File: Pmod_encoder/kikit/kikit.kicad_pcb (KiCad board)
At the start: 2 copper layers, 93.2 x 99.2 mm, 416 parts, among them SW1 SW_SPDT, SW2 RotaryEncoder_Switch

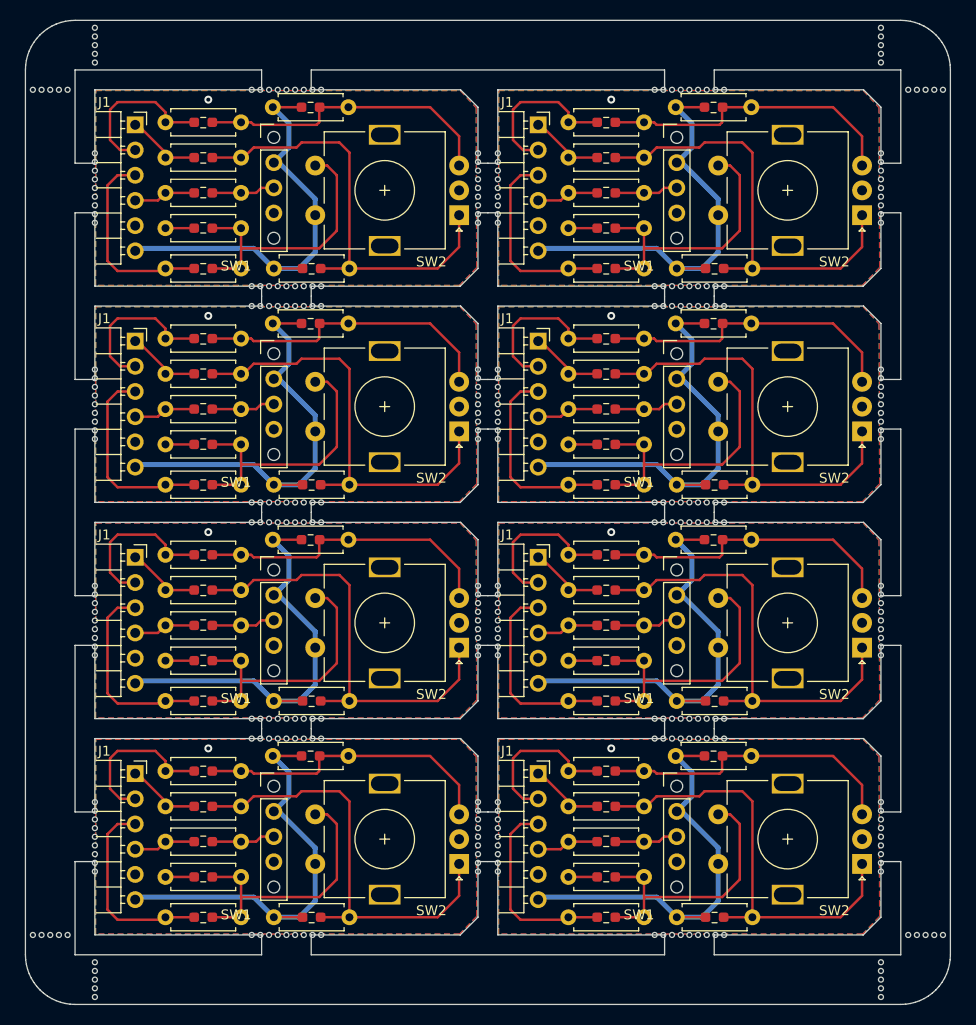
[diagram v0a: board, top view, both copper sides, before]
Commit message: 605
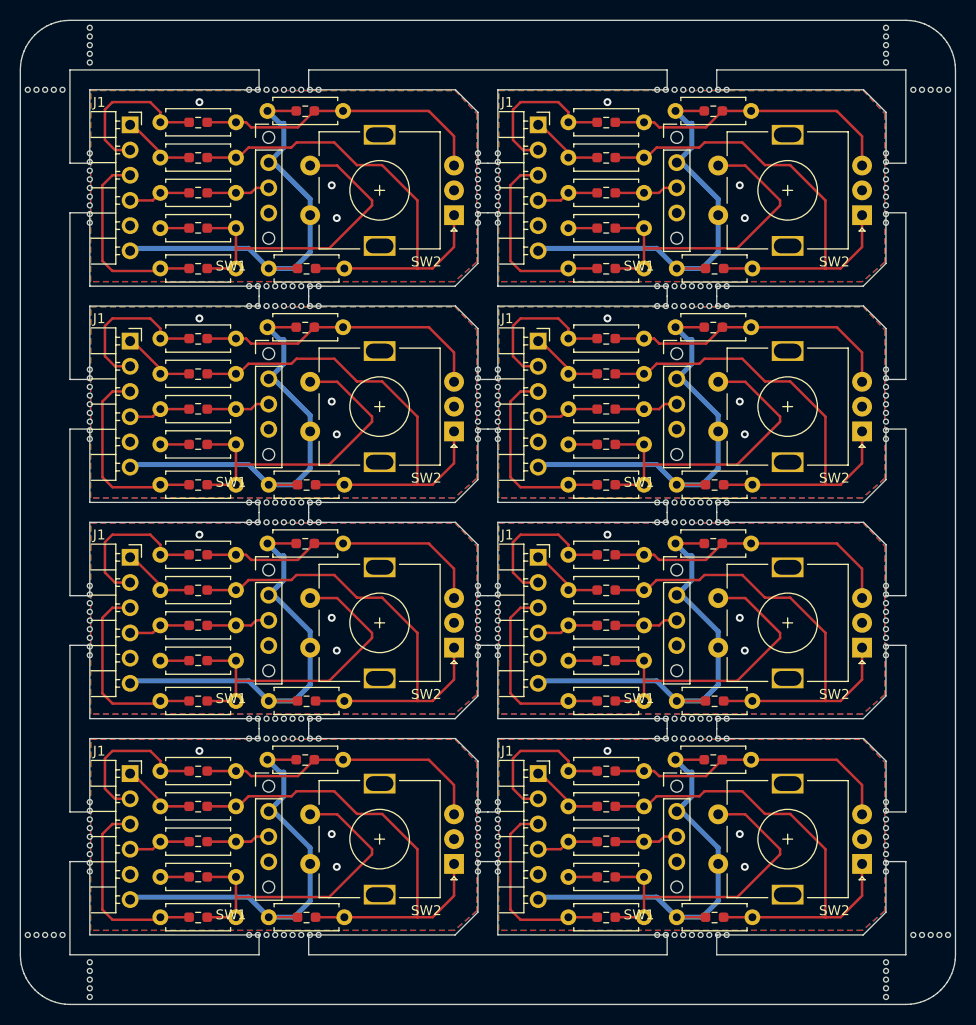
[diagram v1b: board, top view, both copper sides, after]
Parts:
- removed the G*** at (137.6, 37.1)
- removed the G*** at (137.6, 58.9)
- removed the G*** at (137.6, 102.5)
- removed the G*** at (137.6, 80.7)
- removed the J1 at (113.0, 95.9)
- removed the J1 at (113.0, 30.5)
- removed the J1 at (113.0, 52.3)
- removed the J1 at (113.0, 74.1)
- removed the R1 at (123.6, 37.4)
- removed the R1 at (123.6, 81.0)
- removed the R1 at (123.6, 59.2)
- removed the R1 at (123.6, 102.8)
- removed the R2 at (116.0, 95.7)
- removed the R2 at (116.0, 52.1)
- removed the R2 at (116.0, 30.3)
- removed the R2 at (116.0, 73.9)
- removed the R3 at (116.0, 99.2)
- removed the R3 at (116.0, 33.8)
- removed the R3 at (116.0, 55.6)
- removed the R3 at (116.0, 77.4)
- removed the R4 at (116.0, 110.4)
- removed the R4 at (116.0, 88.6)
- removed the R4 at (116.0, 45.0)
- removed the R4 at (116.0, 66.8)
- removed the R5 at (167.4, 28.8)
- removed the R5 at (126.8, 94.1)
- removed the R5 at (126.8, 72.3)
- removed the R5 at (167.4, 72.3)
- removed the R5 at (126.8, 50.5)
- removed the R5 at (167.4, 94.1)
- removed the R5 at (126.8, 28.8)
- removed the R5 at (167.4, 50.5)
- removed the R6 at (123.6, 106.3)
- removed the R6 at (123.6, 84.5)
- removed the R6 at (123.6, 40.9)
- removed the R6 at (123.6, 62.7)
- removed the R7 at (126.9, 45.0)
- removed the R7 at (126.9, 110.4)
- removed the R7 at (126.9, 66.8)
- removed the R7 at (126.9, 88.6)
- removed the REF** at (168.8, 68.6)
- removed the REF** at (124.7, 68.6)
- removed the REF** at (168.8, 27.0)
- removed the REF** at (168.8, 48.8)
- removed the REF** at (147.5, 84.0)
- removed the REF** at (165.3, 27.0)
- removed the REF** at (125.6, 27.0)
- removed the REF** at (147.5, 34.3)
- removed the REF** at (147.5, 77.0)
- removed the REF** at (188.1, 101.4)
- removed the REF** at (172.3, 90.4)
- removed the REF** at (188.1, 38.6)
- removed the REF** at (108.9, 40.4)
- removed the REF** at (128.2, 112.2)
- removed the REF** at (167.1, 68.6)
- removed the REF** at (147.5, 37.8)
- removed the REF** at (188.1, 40.4)
- removed the REF** at (191.7, 112.2)
- removed the REF** at (169.7, 68.6)
- removed the REF** at (126.4, 48.8)
- removed the REF** at (147.5, 104.0)
- removed the REF** at (125.6, 70.6)
- removed the REF** at (165.3, 68.6)
- removed the REF** at (127.3, 112.2)
- removed the REF** at (129.1, 70.6)
- removed the REF** at (172.3, 70.6)
- removed the REF** at (131.7, 27.0)
- removed the REF** at (131.7, 112.2)
- removed the REF** at (166.2, 92.4)
- removed the REF** at (191.7, 27.0)
- removed the REF** at (188.1, 81.4)
- removed the REF** at (108.9, 34.3)
- removed the REF** at (188.1, 56.1)
- removed the REF** at (125.6, 48.8)
- removed the REF** at (102.6, 112.2)
- removed the REF** at (124.7, 27.0)
- removed the REF** at (108.9, 59.6)
- removed the REF** at (108.9, 84.0)
- removed the REF** at (171.4, 48.8)
- removed the REF** at (147.5, 62.2)
- removed the REF** at (147.5, 36.9)
- removed the REF** at (165.3, 92.4)
- removed the REF** at (129.9, 92.4)
- removed the REF** at (188.1, 24.2)
- removed the REF** at (167.9, 46.8)
- removed the REF** at (172.3, 48.8)
- removed the REF** at (188.1, 100.5)
- removed the REF** at (147.5, 61.3)
- removed the REF** at (106.1, 112.2)
- removed the REF** at (128.2, 90.4)
- removed the REF** at (124.7, 112.2)
- removed the REF** at (108.9, 56.9)
- removed the REF** at (165.3, 48.8)
- removed the REF** at (131.7, 90.4)
- removed the REF** at (108.9, 77.0)
- removed the REF** at (147.5, 100.5)
- removed the REF** at (147.5, 59.6)
- removed the REF** at (167.1, 92.4)
- removed the REF** at (166.2, 48.8)
- removed the REF** at (188.1, 118.4)
- removed the REF** at (131.7, 68.6)
- removed the REF** at (124.7, 90.4)
- removed the REF** at (188.1, 62.2)
- removed the REF** at (166.2, 27.0)
- removed the REF** at (108.9, 117.6)
- removed the REF** at (108.9, 57.8)
- removed the REF** at (167.9, 27.0)
- removed the REF** at (147.5, 80.5)
- removed the REF** at (167.9, 48.8)
- removed the REF** at (129.9, 46.8)
- removed the REF** at (128.2, 68.6)
- removed the REF** at (170.6, 92.4)
- removed the REF** at (147.5, 56.9)
- removed the REF** at (147.5, 104.9)
- removed the REF** at (108.9, 101.4)
- removed the REF** at (188.1, 36.0)
- removed the REF** at (147.5, 102.3)
- removed the REF** at (188.1, 104.0)
- removed the REF** at (167.9, 68.6)
- removed the REF** at (171.4, 112.2)
- removed the REF** at (188.1, 84.0)
- removed the REF** at (108.9, 39.5)
- removed the REF** at (125.6, 112.2)
- removed the REF** at (188.1, 82.2)
- removed the REF** at (147.5, 55.2)
- removed the REF** at (129.9, 70.6)
- removed the REF** at (108.9, 78.7)
- removed the REF** at (126.4, 112.2)
- removed the REF** at (167.9, 90.4)
- removed the REF** at (108.9, 36.9)
- removed the REF** at (147.5, 101.4)
- removed the REF** at (125.6, 90.4)
- removed the REF** at (188.1, 83.1)
- removed the REF** at (128.2, 48.8)
- removed the REF** at (188.1, 115.8)
- removed the REF** at (188.1, 105.8)
- removed the REF** at (169.7, 46.8)
- removed the REF** at (168.8, 46.8)
- removed the REF** at (108.9, 115.8)
- removed the REF** at (108.9, 37.8)
- removed the REF** at (108.9, 104.9)
- removed the REF** at (131.7, 48.8)
- removed the REF** at (194.4, 27.0)
- removed the REF** at (147.5, 38.6)
- removed the REF** at (108.9, 24.2)
- removed the REF** at (188.1, 39.5)
- removed the REF** at (147.5, 83.1)
- removed the REF** at (147.5, 99.7)
- removed the REF** at (147.5, 105.8)
- removed the REF** at (108.9, 99.7)
- removed the REF** at (131.7, 46.8)
- removed the REF** at (165.3, 70.6)
- removed the REF** at (108.9, 55.2)
- removed the REF** at (127.3, 68.6)
- removed the REF** at (194.4, 112.2)
- removed the REF** at (108.9, 60.4)
- removed the REF** at (188.1, 99.7)
- removed the REF** at (167.9, 112.2)
- removed the REF** at (105.3, 112.2)
- removed the REF** at (166.2, 46.8)
- removed the REF** at (129.9, 90.4)
- removed the REF** at (129.9, 48.8)
- removed the REF** at (170.6, 48.8)
- removed the REF** at (188.1, 59.6)
- removed the REF** at (168.8, 92.4)
- removed the REF** at (165.3, 90.4)
- removed the REF** at (129.1, 48.8)
- removed the REF** at (166.2, 68.6)
- removed the REF** at (147.5, 36.0)
- removed the REF** at (108.9, 22.5)
- removed the REF** at (129.1, 68.6)
- removed the REF** at (193.5, 27.0)
- removed the REF** at (188.1, 78.7)
- removed the REF** at (108.9, 116.7)
- removed the REF** at (170.6, 112.2)
- removed the REF** at (108.9, 102.3)
- removed the REF** at (108.9, 21.6)
- removed the REF** at (129.9, 27.0)
- removed the REF** at (165.3, 112.2)
- removed the REF** at (167.9, 92.4)
- removed the REF** at (171.4, 68.6)
- removed the REF** at (108.9, 118.4)
- removed the REF** at (130.8, 48.8)
- removed the REF** at (166.2, 70.6)
- removed the REF** at (108.9, 38.6)
- removed the REF** at (108.9, 61.3)
- removed the REF** at (171.4, 70.6)
- removed the REF** at (167.1, 46.8)
- removed the REF** at (188.1, 61.3)
- removed the REF** at (131.7, 70.6)
- removed the REF** at (169.7, 48.8)
- removed the REF** at (128.2, 70.6)
- removed the REF** at (167.9, 70.6)
- removed the REF** at (108.9, 56.1)
- removed the REF** at (108.9, 58.7)
- removed the REF** at (171.4, 92.4)
- removed the REF** at (129.1, 92.4)
- removed the REF** at (130.8, 46.8)
- removed the REF** at (188.1, 117.6)
- removed the REF** at (188.1, 36.9)
- removed the REF** at (168.8, 112.2)
- removed the REF** at (147.5, 60.4)
- removed the REF** at (167.1, 70.6)
- removed the REF** at (108.9, 104.0)
- removed the REF** at (147.5, 40.4)
- removed the REF** at (167.1, 27.0)
- removed the REF** at (188.1, 80.5)
- removed the REF** at (108.9, 100.5)
- removed the REF** at (171.4, 27.0)
- removed the REF** at (172.3, 27.0)
- removed the REF** at (188.1, 98.8)
- removed the REF** at (147.5, 82.2)
- removed the REF** at (188.1, 77.9)
- removed the REF** at (104.4, 112.2)
- removed the REF** at (125.6, 92.4)
- removed the REF** at (147.5, 79.6)
- removed the REF** at (147.5, 103.2)
- removed the REF** at (169.7, 90.4)
- removed the REF** at (126.4, 92.4)
- removed the REF** at (129.9, 112.2)
- removed the REF** at (147.5, 77.9)
- removed the REF** at (108.9, 20.8)
- removed the REF** at (188.1, 79.6)
- removed the REF** at (129.1, 27.0)
- removed the REF** at (130.8, 92.4)
- removed the REF** at (147.5, 81.4)
- removed the REF** at (108.9, 114.9)
- removed the REF** at (192.6, 112.2)
- removed the REF** at (130.8, 27.0)
- removed the REF** at (188.1, 102.3)
- removed the REF** at (127.3, 46.8)
- removed the REF** at (130.8, 112.2)
- removed the REF** at (147.5, 39.5)
- removed the REF** at (170.6, 27.0)
- removed the REF** at (108.9, 36.0)
- removed the REF** at (126.4, 27.0)
- removed the REF** at (188.1, 57.8)
- removed the REF** at (167.1, 48.8)
- removed the REF** at (188.1, 33.4)
- removed the REF** at (104.4, 27.0)
- removed the REF** at (129.9, 68.6)
- removed the REF** at (131.7, 92.4)
- removed the REF** at (127.3, 48.8)
- removed the REF** at (147.5, 58.7)
- removed the REF** at (127.3, 27.0)
- removed the REF** at (170.6, 90.4)
- removed the REF** at (171.4, 90.4)
- removed the REF** at (103.5, 112.2)
- removed the REF** at (166.2, 112.2)
- removed the REF** at (170.6, 68.6)
- removed the REF** at (129.1, 112.2)
- removed the REF** at (108.9, 33.4)
- removed the REF** at (126.4, 46.8)
- removed the REF** at (130.8, 70.6)
- removed the REF** at (188.1, 23.4)
- removed the REF** at (126.4, 90.4)
- removed the REF** at (108.9, 81.4)
- removed the REF** at (108.9, 82.2)
- removed the REF** at (147.5, 35.1)
- removed the REF** at (170.6, 70.6)
- removed the REF** at (108.9, 105.8)
- removed the REF** at (188.1, 77.0)
- removed the REF** at (188.1, 35.1)
- removed the REF** at (108.9, 23.4)
- removed the REF** at (188.1, 22.5)
- removed the REF** at (166.2, 90.4)
- removed the REF** at (124.7, 48.8)
- removed the REF** at (165.3, 46.8)
- removed the REF** at (127.3, 70.6)
- removed the REF** at (188.1, 21.6)
- removed the REF** at (190.9, 112.2)
- removed the REF** at (171.4, 46.8)
- removed the REF** at (188.1, 34.3)
- removed the REF** at (188.1, 116.7)
- removed the REF** at (102.6, 27.0)
- removed the REF** at (172.3, 112.2)
- removed the REF** at (124.7, 92.4)
- removed the REF** at (168.8, 90.4)
- removed the REF** at (108.9, 35.1)
- removed the REF** at (129.1, 46.8)
- removed the REF** at (167.1, 90.4)
- removed the REF** at (125.6, 68.6)
- removed the REF** at (124.7, 70.6)
- removed the REF** at (108.9, 79.6)
- removed the REF** at (126.4, 68.6)
- removed the REF** at (147.5, 78.7)
- removed the REF** at (147.5, 56.1)
- removed the REF** at (126.4, 70.6)
- removed the REF** at (188.1, 56.9)
- removed the REF** at (168.8, 70.6)
- removed the REF** at (108.9, 98.8)
- removed the REF** at (188.1, 37.8)
- removed the REF** at (108.9, 80.5)
- removed the REF** at (105.3, 27.0)
- removed the REF** at (188.1, 55.2)
- removed the REF** at (172.3, 46.8)
- removed the REF** at (147.5, 98.8)
- removed the REF** at (124.7, 46.8)
- removed the REF** at (192.6, 27.0)
- removed the REF** at (127.3, 92.4)
- removed the REF** at (188.1, 20.8)
- removed the REF** at (172.3, 68.6)
- removed the REF** at (129.1, 90.4)
- removed the REF** at (127.3, 90.4)
- removed the REF** at (169.7, 92.4)
- removed the REF** at (147.5, 57.8)
- removed the REF** at (172.3, 92.4)
- removed the REF** at (108.9, 83.1)
- removed the REF** at (190.9, 27.0)
- removed the REF** at (147.5, 33.4)
- removed the REF** at (170.6, 46.8)
- removed the REF** at (188.1, 58.7)
- removed the REF** at (103.5, 27.0)
- removed the REF** at (130.8, 68.6)
- removed the REF** at (188.1, 103.2)
- removed the REF** at (128.2, 27.0)
- removed the REF** at (108.9, 62.2)
- removed the REF** at (108.9, 77.9)
- removed the REF** at (169.7, 70.6)
- removed the REF** at (188.1, 60.4)
- removed the REF** at (108.9, 103.2)
- removed the REF** at (167.1, 112.2)
- removed the REF** at (130.8, 90.4)
- removed the REF** at (128.2, 92.4)
- removed the REF** at (128.2, 46.8)
- removed the REF** at (193.5, 112.2)
- removed the REF** at (125.6, 46.8)
- removed the REF** at (169.7, 27.0)
- removed the REF** at (169.7, 112.2)
- removed the REF** at (106.1, 27.0)
- removed the REF** at (188.1, 104.9)
- removed the REF** at (188.1, 114.9)
- removed the SW1 at (126.9, 53.6)
- removed the SW1 at (126.9, 97.2)
- removed the SW1 at (126.9, 31.8)
- removed the SW1 at (126.9, 75.4)
- removed the SW2 at (145.6, 61.4)
- removed the SW2 at (145.6, 39.6)
- removed the SW2 at (145.6, 83.2)
- removed the SW2 at (145.6, 105.0)
- added G***: LOGO, Library:yagamo_12mm, B.Cu at (137.1, 58.9)
- added G***: LOGO, Library:yagamo_12mm, B.Cu at (137.1, 102.5)
- added G***: LOGO, Library:yagamo_12mm, B.Cu at (137.1, 37.1)
- added G***: LOGO, Library:yagamo_12mm, B.Cu at (137.1, 80.7)
- added J1: ~, Library:Pmod6, F.Cu at (112.4, 74.1)
- added J1: ~, Library:Pmod6, F.Cu at (112.4, 52.3)
- added J1: ~, Library:Pmod6, F.Cu at (112.4, 30.5)
- added J1: ~, Library:Pmod6, F.Cu at (112.4, 95.9)
- added R1: 4.7k, Library:Resistor_SMD_THT, F.Cu at (123.1, 81.0)
- added R1: 4.7k, Library:Resistor_SMD_THT, F.Cu at (123.1, 102.8)
- added R1: 4.7k, Library:Resistor_SMD_THT, F.Cu at (123.1, 59.2)
- added R1: 4.7k, Library:Resistor_SMD_THT, F.Cu at (123.1, 37.4)
- added R2: 4.7k, Library:Resistor_SMD_THT, F.Cu at (115.5, 52.1)
- added R2: 4.7k, Library:Resistor_SMD_THT, F.Cu at (115.5, 73.9)
- added R2: 4.7k, Library:Resistor_SMD_THT, F.Cu at (115.5, 95.7)
- added R2: 4.7k, Library:Resistor_SMD_THT, F.Cu at (115.5, 30.3)
- added R3: 4.7k, Library:Resistor_SMD_THT, F.Cu at (115.5, 55.6)
- added R3: 4.7k, Library:Resistor_SMD_THT, F.Cu at (115.5, 77.4)
- added R3: 4.7k, Library:Resistor_SMD_THT, F.Cu at (115.5, 33.8)
- added R3: 4.7k, Library:Resistor_SMD_THT, F.Cu at (115.5, 99.2)
- added R4: 4.7k, Library:Resistor_SMD_THT, F.Cu at (115.5, 110.4)
- added R4: 4.7k, Library:Resistor_SMD_THT, F.Cu at (115.5, 88.6)
- added R4: 4.7k, Library:Resistor_SMD_THT, F.Cu at (115.5, 66.8)
- added R4: 4.7k, Library:Resistor_SMD_THT, F.Cu at (115.5, 45.0)
- added R5: 4.7k, Library:Resistor_SMD_THT, F.Cu at (126.3, 94.5)
- added R5: 4.7k, Library:Resistor_SMD_THT, F.Cu at (167.4, 94.5)
- added R5: 4.7k, Library:Resistor_SMD_THT, F.Cu at (167.4, 50.9)
- added R5: 4.7k, Library:Resistor_SMD_THT, F.Cu at (126.3, 29.1)
- added R5: 4.7k, Library:Resistor_SMD_THT, F.Cu at (126.3, 50.9)
- added R5: 4.7k, Library:Resistor_SMD_THT, F.Cu at (167.4, 29.1)
- added R5: 4.7k, Library:Resistor_SMD_THT, F.Cu at (126.3, 72.7)
- added R5: 4.7k, Library:Resistor_SMD_THT, F.Cu at (167.4, 72.7)
- added R6: 4.7k, Library:Resistor_SMD_THT, F.Cu at (123.1, 84.5)
- added R6: 4.7k, Library:Resistor_SMD_THT, F.Cu at (123.1, 40.9)
- added R6: 4.7k, Library:Resistor_SMD_THT, F.Cu at (123.1, 106.3)
- added R6: 4.7k, Library:Resistor_SMD_THT, F.Cu at (123.1, 62.7)
- added R7: 4.7k, Library:Resistor_SMD_THT, F.Cu at (126.4, 88.6)
- added R7: 4.7k, Library:Resistor_SMD_THT, F.Cu at (126.4, 66.8)
- added R7: 4.7k, Library:Resistor_SMD_THT, F.Cu at (126.4, 45.0)
- added R7: 4.7k, Library:Resistor_SMD_THT, F.Cu at (126.4, 110.4)
- added REF**: NPTH, NPTH, F.Cu at (108.4, 23.4)
- added REF**: NPTH, NPTH, F.Cu at (188.6, 99.7)
- added REF**: NPTH, NPTH, F.Cu at (103.0, 112.2)
- added REF**: NPTH, NPTH, F.Cu at (188.6, 105.8)
- added REF**: NPTH, NPTH, F.Cu at (108.4, 104.0)
- added REF**: NPTH, NPTH, F.Cu at (104.8, 27.0)
- added REF**: NPTH, NPTH, F.Cu at (188.6, 104.0)
- added REF**: NPTH, NPTH, F.Cu at (188.6, 60.4)
- added REF**: NPTH, NPTH, F.Cu at (166.4, 70.6)
- added REF**: NPTH, NPTH, F.Cu at (103.9, 112.2)
- added REF**: NPTH, NPTH, F.Cu at (169.9, 92.4)
- added REF**: NPTH, NPTH, F.Cu at (188.6, 100.5)
- added REF**: NPTH, NPTH, F.Cu at (129.7, 92.4)
- added REF**: NPTH, NPTH, F.Cu at (165.6, 112.2)
- added REF**: NPTH, NPTH, F.Cu at (108.4, 83.1)
- added REF**: NPTH, NPTH, F.Cu at (165.6, 92.4)
- added REF**: NPTH, NPTH, F.Cu at (108.4, 38.6)
- added REF**: NPTH, NPTH, F.Cu at (191.4, 27.0)
- added REF**: NPTH, NPTH, F.Cu at (165.6, 68.6)
- added REF**: NPTH, NPTH, F.Cu at (188.6, 104.9)
- added REF**: NPTH, NPTH, F.Cu at (169.1, 90.4)
- added REF**: NPTH, NPTH, F.Cu at (170.8, 46.8)
- added REF**: NPTH, NPTH, F.Cu at (170.8, 27.0)
- added REF**: NPTH, NPTH, F.Cu at (130.6, 48.8)
- added REF**: NPTH, NPTH, F.Cu at (108.4, 81.4)
- added REF**: NPTH, NPTH, F.Cu at (188.6, 103.2)
- added REF**: NPTH, NPTH, F.Cu at (168.2, 90.4)
- added REF**: NPTH, NPTH, F.Cu at (108.4, 77.0)
- added REF**: NPTH, NPTH, F.Cu at (147.5, 36.0)
- added REF**: NPTH, NPTH, F.Cu at (167.3, 48.8)
- added REF**: NPTH, NPTH, F.Cu at (108.4, 40.4)
- added REF**: NPTH, NPTH, F.Cu at (193.1, 112.2)
- added REF**: NPTH, NPTH, F.Cu at (172.6, 27.0)
- added REF**: NPTH, NPTH, F.Cu at (188.6, 33.4)
- added REF**: NPTH, NPTH, F.Cu at (129.7, 27.0)
- added REF**: NPTH, NPTH, F.Cu at (125.3, 68.6)
- added REF**: NPTH, NPTH, F.Cu at (170.8, 92.4)
- added REF**: NPTH, NPTH, F.Cu at (125.3, 90.4)
- added REF**: NPTH, NPTH, F.Cu at (188.6, 83.1)
- added REF**: NPTH, NPTH, F.Cu at (127.1, 70.6)
- added REF**: NPTH, NPTH, F.Cu at (147.5, 105.8)
- added REF**: NPTH, NPTH, F.Cu at (127.9, 46.8)
- added REF**: NPTH, NPTH, F.Cu at (167.3, 68.6)
- added REF**: NPTH, NPTH, F.Cu at (125.3, 27.0)
- added REF**: NPTH, NPTH, F.Cu at (172.6, 68.6)
- added REF**: NPTH, NPTH, F.Cu at (128.8, 70.6)
- added REF**: NPTH, NPTH, F.Cu at (124.4, 92.4)
- added REF**: NPTH, NPTH, F.Cu at (126.2, 70.6)
- added REF**: NPTH, NPTH, F.Cu at (126.2, 112.2)
- added REF**: NPTH, NPTH, F.Cu at (108.4, 78.7)
- added REF**: NPTH, NPTH, F.Cu at (188.6, 117.6)
- added REF**: NPTH, NPTH, F.Cu at (108.4, 61.3)
- added REF**: NPTH, NPTH, F.Cu at (124.4, 90.4)
- added REF**: NPTH, NPTH, F.Cu at (188.6, 78.7)
- added REF**: NPTH, NPTH, F.Cu at (169.9, 68.6)
- added REF**: NPTH, NPTH, F.Cu at (169.1, 48.8)
- added REF**: NPTH, NPTH, F.Cu at (131.4, 70.6)
- added REF**: NPTH, NPTH, F.Cu at (130.6, 90.4)
- added REF**: NPTH, NPTH, F.Cu at (172.6, 48.8)
- added REF**: NPTH, NPTH, F.Cu at (188.6, 23.4)
- added REF**: NPTH, NPTH, F.Cu at (125.3, 92.4)
- added REF**: NPTH, NPTH, F.Cu at (127.9, 27.0)
- added REF**: NPTH, NPTH, F.Cu at (127.1, 68.6)
- added REF**: NPTH, NPTH, F.Cu at (128.8, 27.0)
- added REF**: NPTH, NPTH, F.Cu at (168.2, 92.4)
- added REF**: NPTH, NPTH, F.Cu at (188.6, 82.2)
- added REF**: NPTH, NPTH, F.Cu at (108.4, 56.1)
- added REF**: NPTH, NPTH, F.Cu at (171.7, 68.6)
- added REF**: NPTH, NPTH, F.Cu at (130.6, 68.6)
- added REF**: NPTH, NPTH, F.Cu at (166.4, 90.4)
- added REF**: NPTH, NPTH, F.Cu at (188.6, 62.2)
- added REF**: NPTH, NPTH, F.Cu at (147.5, 77.0)
- added REF**: NPTH, NPTH, F.Cu at (108.4, 20.8)
- added REF**: NPTH, NPTH, F.Cu at (147.5, 57.8)
- added REF**: NPTH, NPTH, F.Cu at (105.6, 27.0)
- added REF**: NPTH, NPTH, F.Cu at (147.5, 99.7)
- added REF**: NPTH, NPTH, F.Cu at (147.5, 83.1)
- added REF**: NPTH, NPTH, F.Cu at (108.4, 82.2)
- added REF**: NPTH, NPTH, F.Cu at (188.6, 59.6)
- added REF**: NPTH, NPTH, F.Cu at (127.1, 46.8)
- added REF**: NPTH, NPTH, F.Cu at (108.4, 117.6)
- added REF**: NPTH, NPTH, F.Cu at (188.6, 77.9)
- added REF**: NPTH, NPTH, F.Cu at (172.6, 92.4)
- added REF**: NPTH, NPTH, F.Cu at (104.8, 112.2)
- added REF**: NPTH, NPTH, F.Cu at (188.6, 57.8)
- added REF**: NPTH, NPTH, F.Cu at (168.2, 70.6)
- added REF**: NPTH, NPTH, F.Cu at (166.4, 92.4)
- added REF**: NPTH, NPTH, F.Cu at (188.6, 98.8)
- added REF**: NPTH, NPTH, F.Cu at (103.0, 27.0)
- added REF**: NPTH, NPTH, F.Cu at (188.6, 101.4)
- added REF**: NPTH, NPTH, F.Cu at (168.2, 68.6)
- added REF**: NPTH, NPTH, F.Cu at (188.6, 37.8)
- added REF**: NPTH, NPTH, F.Cu at (147.5, 79.6)
- added REF**: NPTH, NPTH, F.Cu at (124.4, 70.6)
- added REF**: NPTH, NPTH, F.Cu at (194.9, 112.2)
- added REF**: NPTH, NPTH, F.Cu at (127.1, 48.8)
- added REF**: NPTH, NPTH, F.Cu at (108.4, 105.8)
- added REF**: NPTH, NPTH, F.Cu at (147.5, 61.3)
- added REF**: NPTH, NPTH, F.Cu at (170.8, 90.4)
- added REF**: NPTH, NPTH, F.Cu at (171.7, 27.0)
- added REF**: NPTH, NPTH, F.Cu at (124.4, 68.6)
- added REF**: NPTH, NPTH, F.Cu at (147.5, 34.3)
- added REF**: NPTH, NPTH, F.Cu at (108.4, 22.5)
- added REF**: NPTH, NPTH, F.Cu at (188.6, 35.1)
- added REF**: NPTH, NPTH, F.Cu at (147.5, 81.4)
- added REF**: NPTH, NPTH, F.Cu at (102.1, 112.2)
- added REF**: NPTH, NPTH, F.Cu at (169.1, 27.0)
- added REF**: NPTH, NPTH, F.Cu at (192.2, 27.0)
- added REF**: NPTH, NPTH, F.Cu at (108.4, 116.7)
- added REF**: NPTH, NPTH, F.Cu at (147.5, 33.4)
- added REF**: NPTH, NPTH, F.Cu at (169.1, 46.8)
- added REF**: NPTH, NPTH, F.Cu at (188.6, 36.9)
- added REF**: NPTH, NPTH, F.Cu at (166.4, 68.6)
- added REF**: NPTH, NPTH, F.Cu at (108.4, 56.9)
- added REF**: NPTH, NPTH, F.Cu at (125.3, 46.8)
- added REF**: NPTH, NPTH, F.Cu at (129.7, 70.6)
- added REF**: NPTH, NPTH, F.Cu at (165.6, 27.0)
- added REF**: NPTH, NPTH, F.Cu at (124.4, 48.8)
- added REF**: NPTH, NPTH, F.Cu at (193.1, 27.0)
- added REF**: NPTH, NPTH, F.Cu at (188.6, 56.9)
- added REF**: NPTH, NPTH, F.Cu at (188.6, 114.9)
- added REF**: NPTH, NPTH, F.Cu at (108.4, 84.0)
- added REF**: NPTH, NPTH, F.Cu at (128.8, 68.6)
- added REF**: NPTH, NPTH, F.Cu at (188.6, 79.6)
- added REF**: NPTH, NPTH, F.Cu at (169.9, 27.0)
- added REF**: NPTH, NPTH, F.Cu at (128.8, 46.8)
- added REF**: NPTH, NPTH, F.Cu at (147.5, 77.9)
- added REF**: NPTH, NPTH, F.Cu at (130.6, 27.0)
- added REF**: NPTH, NPTH, F.Cu at (188.6, 116.7)
- added REF**: NPTH, NPTH, F.Cu at (147.5, 104.9)
- added REF**: NPTH, NPTH, F.Cu at (194.0, 112.2)
- added REF**: NPTH, NPTH, F.Cu at (170.8, 70.6)
- added REF**: NPTH, NPTH, F.Cu at (166.4, 48.8)
- added REF**: NPTH, NPTH, F.Cu at (108.4, 59.6)
- added REF**: NPTH, NPTH, F.Cu at (191.4, 112.2)
- added REF**: NPTH, NPTH, F.Cu at (125.3, 112.2)
- added REF**: NPTH, NPTH, F.Cu at (167.3, 112.2)
- added REF**: NPTH, NPTH, F.Cu at (171.7, 90.4)
- added REF**: NPTH, NPTH, F.Cu at (167.3, 92.4)
- added REF**: NPTH, NPTH, F.Cu at (147.5, 56.1)
- added REF**: NPTH, NPTH, F.Cu at (127.1, 90.4)
- added REF**: NPTH, NPTH, F.Cu at (169.1, 68.6)
- added REF**: NPTH, NPTH, F.Cu at (108.4, 118.4)
- added REF**: NPTH, NPTH, F.Cu at (167.3, 27.0)
- added REF**: NPTH, NPTH, F.Cu at (108.4, 21.6)
- added REF**: NPTH, NPTH, F.Cu at (147.5, 60.4)
- added REF**: NPTH, NPTH, F.Cu at (147.5, 40.4)
- added REF**: NPTH, NPTH, F.Cu at (127.9, 48.8)
- added REF**: NPTH, NPTH, F.Cu at (108.4, 79.6)
- added REF**: NPTH, NPTH, F.Cu at (147.5, 100.5)
- added REF**: NPTH, NPTH, F.Cu at (188.6, 61.3)
- added REF**: NPTH, NPTH, F.Cu at (188.6, 20.8)
- added REF**: NPTH, NPTH, F.Cu at (167.3, 90.4)
- added REF**: NPTH, NPTH, F.Cu at (108.4, 33.4)
- added REF**: NPTH, NPTH, F.Cu at (108.4, 55.2)
- added REF**: NPTH, NPTH, F.Cu at (126.2, 48.8)
- added REF**: NPTH, NPTH, F.Cu at (188.6, 39.5)
- added REF**: NPTH, NPTH, F.Cu at (188.6, 102.3)
- added REF**: NPTH, NPTH, F.Cu at (147.5, 55.2)
- added REF**: NPTH, NPTH, F.Cu at (128.8, 112.2)
- added REF**: NPTH, NPTH, F.Cu at (170.8, 112.2)
- added REF**: NPTH, NPTH, F.Cu at (172.6, 46.8)
- added REF**: NPTH, NPTH, F.Cu at (147.5, 101.4)
- added REF**: NPTH, NPTH, F.Cu at (188.6, 77.0)
- added REF**: NPTH, NPTH, F.Cu at (124.4, 46.8)
- added REF**: NPTH, NPTH, F.Cu at (192.2, 112.2)
- added REF**: NPTH, NPTH, F.Cu at (169.9, 46.8)
- added REF**: NPTH, NPTH, F.Cu at (108.4, 103.2)
- added REF**: NPTH, NPTH, F.Cu at (194.9, 27.0)
- added REF**: NPTH, NPTH, F.Cu at (130.6, 70.6)
- added REF**: NPTH, NPTH, F.Cu at (171.7, 46.8)
- added REF**: NPTH, NPTH, F.Cu at (131.4, 48.8)
- added REF**: NPTH, NPTH, F.Cu at (126.2, 68.6)
- added REF**: NPTH, NPTH, F.Cu at (165.6, 90.4)
- added REF**: NPTH, NPTH, F.Cu at (188.6, 36.0)
- added REF**: NPTH, NPTH, F.Cu at (169.1, 92.4)
- added REF**: NPTH, NPTH, F.Cu at (127.9, 112.2)
- added REF**: NPTH, NPTH, F.Cu at (129.7, 68.6)
- added REF**: NPTH, NPTH, F.Cu at (147.5, 104.0)
- added REF**: NPTH, NPTH, F.Cu at (188.6, 115.8)
- added REF**: NPTH, NPTH, F.Cu at (127.1, 112.2)
- added REF**: NPTH, NPTH, F.Cu at (168.2, 48.8)
- added REF**: NPTH, NPTH, F.Cu at (170.8, 48.8)
- added REF**: NPTH, NPTH, F.Cu at (169.1, 112.2)
- added REF**: NPTH, NPTH, F.Cu at (169.1, 70.6)
- added REF**: NPTH, NPTH, F.Cu at (188.6, 34.3)
- added REF**: NPTH, NPTH, F.Cu at (188.6, 38.6)
- added REF**: NPTH, NPTH, F.Cu at (127.9, 70.6)
- added REF**: NPTH, NPTH, F.Cu at (169.9, 70.6)
- added REF**: NPTH, NPTH, F.Cu at (128.8, 92.4)
- added REF**: NPTH, NPTH, F.Cu at (108.4, 39.5)
- added REF**: NPTH, NPTH, F.Cu at (128.8, 48.8)
- added REF**: NPTH, NPTH, F.Cu at (147.5, 37.8)
- added REF**: NPTH, NPTH, F.Cu at (188.6, 118.4)
- added REF**: NPTH, NPTH, F.Cu at (166.4, 112.2)
- added REF**: NPTH, NPTH, F.Cu at (167.3, 70.6)
- added REF**: NPTH, NPTH, F.Cu at (188.6, 40.4)
- added REF**: NPTH, NPTH, F.Cu at (126.2, 92.4)
- added REF**: NPTH, NPTH, F.Cu at (188.6, 80.5)
- added REF**: NPTH, NPTH, F.Cu at (188.6, 24.2)
- added REF**: NPTH, NPTH, F.Cu at (131.4, 92.4)
- added REF**: NPTH, NPTH, F.Cu at (147.5, 102.3)
- added REF**: NPTH, NPTH, F.Cu at (125.3, 48.8)
- added REF**: NPTH, NPTH, F.Cu at (188.6, 56.1)
- added REF**: NPTH, NPTH, F.Cu at (105.6, 112.2)
- added REF**: NPTH, NPTH, F.Cu at (147.5, 39.5)
- added REF**: NPTH, NPTH, F.Cu at (147.5, 56.9)
- added REF**: NPTH, NPTH, F.Cu at (188.6, 55.2)
- added REF**: NPTH, NPTH, F.Cu at (147.5, 35.1)
- added REF**: NPTH, NPTH, F.Cu at (188.6, 21.6)
- added REF**: NPTH, NPTH, F.Cu at (126.2, 46.8)
- added REF**: NPTH, NPTH, F.Cu at (130.6, 46.8)
- added REF**: NPTH, NPTH, F.Cu at (129.7, 48.8)
- added REF**: NPTH, NPTH, F.Cu at (194.0, 27.0)
- added REF**: NPTH, NPTH, F.Cu at (102.1, 27.0)
- added REF**: NPTH, NPTH, F.Cu at (108.4, 57.8)
- added REF**: NPTH, NPTH, F.Cu at (125.3, 70.6)
- added REF**: NPTH, NPTH, F.Cu at (108.4, 60.4)
- added REF**: NPTH, NPTH, F.Cu at (131.4, 27.0)
- added REF**: NPTH, NPTH, F.Cu at (103.9, 27.0)
- added REF**: NPTH, NPTH, F.Cu at (108.4, 98.8)
- added REF**: NPTH, NPTH, F.Cu at (126.2, 27.0)
- added REF**: NPTH, NPTH, F.Cu at (170.8, 68.6)
- added REF**: NPTH, NPTH, F.Cu at (188.6, 22.5)
- added REF**: NPTH, NPTH, F.Cu at (171.7, 70.6)
- added REF**: NPTH, NPTH, F.Cu at (108.4, 36.9)
- added REF**: NPTH, NPTH, F.Cu at (147.5, 82.2)
- added REF**: NPTH, NPTH, F.Cu at (131.4, 90.4)
- added REF**: NPTH, NPTH, F.Cu at (127.9, 68.6)
- added REF**: NPTH, NPTH, F.Cu at (169.9, 48.8)
- added REF**: NPTH, NPTH, F.Cu at (131.4, 68.6)
- added REF**: NPTH, NPTH, F.Cu at (108.4, 80.5)
- added REF**: NPTH, NPTH, F.Cu at (108.4, 62.2)
- added REF**: NPTH, NPTH, F.Cu at (188.6, 81.4)
- added REF**: NPTH, NPTH, F.Cu at (108.4, 35.1)
- added REF**: NPTH, NPTH, F.Cu at (127.1, 92.4)
- added REF**: NPTH, NPTH, F.Cu at (108.4, 100.5)
- added REF**: NPTH, NPTH, F.Cu at (147.5, 62.2)
- added REF**: NPTH, NPTH, F.Cu at (128.8, 90.4)
- added REF**: NPTH, NPTH, F.Cu at (147.5, 38.6)
- added REF**: NPTH, NPTH, F.Cu at (147.5, 80.5)
- added REF**: NPTH, NPTH, F.Cu at (108.4, 102.3)
- added REF**: NPTH, NPTH, F.Cu at (169.9, 112.2)
- added REF**: NPTH, NPTH, F.Cu at (168.2, 46.8)
- added REF**: NPTH, NPTH, F.Cu at (147.5, 58.7)
- added REF**: NPTH, NPTH, F.Cu at (108.4, 114.9)
- added REF**: NPTH, NPTH, F.Cu at (147.5, 84.0)
- added REF**: NPTH, NPTH, F.Cu at (172.6, 90.4)
- added REF**: NPTH, NPTH, F.Cu at (165.6, 48.8)
- added REF**: NPTH, NPTH, F.Cu at (165.6, 70.6)
- added REF**: NPTH, NPTH, F.Cu at (108.4, 99.7)
- added REF**: NPTH, NPTH, F.Cu at (165.6, 46.8)
- added REF**: NPTH, NPTH, F.Cu at (171.7, 92.4)
- added REF**: NPTH, NPTH, F.Cu at (147.5, 98.8)
- added REF**: NPTH, NPTH, F.Cu at (166.4, 46.8)
- added REF**: NPTH, NPTH, F.Cu at (108.4, 24.2)
- added REF**: NPTH, NPTH, F.Cu at (127.9, 92.4)
- added REF**: NPTH, NPTH, F.Cu at (130.6, 92.4)
- added REF**: NPTH, NPTH, F.Cu at (108.4, 104.9)
- added REF**: NPTH, NPTH, F.Cu at (147.5, 36.9)
- added REF**: NPTH, NPTH, F.Cu at (147.5, 59.6)
- added REF**: NPTH, NPTH, F.Cu at (171.7, 48.8)
- added REF**: NPTH, NPTH, F.Cu at (171.7, 112.2)
- added REF**: NPTH, NPTH, F.Cu at (168.2, 112.2)
- added REF**: NPTH, NPTH, F.Cu at (124.4, 112.2)
- added REF**: NPTH, NPTH, F.Cu at (131.4, 46.8)
- added REF**: NPTH, NPTH, F.Cu at (108.4, 36.0)
- added REF**: NPTH, NPTH, F.Cu at (130.6, 112.2)
- added REF**: NPTH, NPTH, F.Cu at (169.9, 90.4)
- added REF**: NPTH, NPTH, F.Cu at (166.4, 27.0)
- added REF**: NPTH, NPTH, F.Cu at (108.4, 115.8)
- added REF**: NPTH, NPTH, F.Cu at (129.7, 90.4)
- added REF**: NPTH, NPTH, F.Cu at (129.7, 46.8)
- added REF**: NPTH, NPTH, F.Cu at (108.4, 34.3)
- added REF**: NPTH, NPTH, F.Cu at (108.4, 37.8)
- added REF**: NPTH, NPTH, F.Cu at (108.4, 101.4)
- added REF**: NPTH, NPTH, F.Cu at (167.3, 46.8)
- added REF**: NPTH, NPTH, F.Cu at (188.6, 84.0)
- added REF**: NPTH, NPTH, F.Cu at (172.6, 70.6)
- added REF**: NPTH, NPTH, F.Cu at (108.4, 58.7)
- added REF**: NPTH, NPTH, F.Cu at (127.9, 90.4)
- added REF**: NPTH, NPTH, F.Cu at (129.7, 112.2)
- added REF**: NPTH, NPTH, F.Cu at (127.1, 27.0)
- added REF**: NPTH, NPTH, F.Cu at (188.6, 58.7)
- added REF**: NPTH, NPTH, F.Cu at (172.6, 112.2)
- added REF**: NPTH, NPTH, F.Cu at (168.2, 27.0)
- added REF**: NPTH, NPTH, F.Cu at (126.2, 90.4)
- added REF**: NPTH, NPTH, F.Cu at (108.4, 77.9)
- added REF**: NPTH, NPTH, F.Cu at (124.4, 27.0)
- added REF**: NPTH, NPTH, F.Cu at (131.4, 112.2)
- added REF**: NPTH, NPTH, F.Cu at (147.5, 103.2)
- added REF**: NPTH, NPTH, F.Cu at (147.5, 78.7)
- added SW1: SW_SPDT, Connector_PinHeader_2.54mm:PinHeader_1x05_P2.54mm_Vertical, F.Cu at (126.4, 53.6)
- added SW1: SW_SPDT, Connector_PinHeader_2.54mm:PinHeader_1x05_P2.54mm_Vertical, F.Cu at (126.4, 31.8)
- added SW1: SW_SPDT, Connector_PinHeader_2.54mm:PinHeader_1x05_P2.54mm_Vertical, F.Cu at (126.4, 97.2)
- added SW1: SW_SPDT, Connector_PinHeader_2.54mm:PinHeader_1x05_P2.54mm_Vertical, F.Cu at (126.4, 75.4)
- added SW2: RotaryEncoder_Switch, Rotary_Encoder:RotaryEncoder_Alps_EC11E-Switch_Vertical_H20mm, F.Cu at (145.1, 61.4)
- added SW2: RotaryEncoder_Switch, Rotary_Encoder:RotaryEncoder_Alps_EC11E-Switch_Vertical_H20mm, F.Cu at (145.1, 105.0)
- added SW2: RotaryEncoder_Switch, Rotary_Encoder:RotaryEncoder_Alps_EC11E-Switch_Vertical_H20mm, F.Cu at (145.1, 83.2)
- added SW2: RotaryEncoder_Switch, Rotary_Encoder:RotaryEncoder_Alps_EC11E-Switch_Vertical_H20mm, F.Cu at (145.1, 39.6)
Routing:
- net Board_7-Net-(R4-Pad2): track 28.3 -> 33.4 mm
- net Board_5-Net-(R4-Pad2): track 28.3 -> 33.4 mm
- net Board_1-Net-(R4-Pad2): track 28.3 -> 33.4 mm
- net Board_3-Net-(R4-Pad2): track 28.3 -> 33.4 mm
- net Board_6-Net-(R4-Pad2): track 28.3 -> 33.4 mm
- net Board_0-Net-(R4-Pad2): track 28.3 -> 33.4 mm
- net Board_4-Net-(R4-Pad2): track 28.3 -> 33.4 mm
- net Board_2-Net-(R4-Pad2): track 28.3 -> 33.4 mm
- net Board_7-Net-(R3-Pad2): track 44.7 -> 49.3 mm
- net Board_6-Net-(R3-Pad2): track 44.7 -> 49.3 mm
- net Board_3-Net-(R3-Pad2): track 44.7 -> 49.3 mm
- net Board_1-Net-(R3-Pad2): track 44.7 -> 49.3 mm
- net Board_5-Net-(R3-Pad2): track 44.7 -> 49.3 mm
- net Board_4-Net-(R3-Pad2): track 44.7 -> 49.3 mm
- net Board_2-Net-(R3-Pad2): track 44.7 -> 49.3 mm
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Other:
- board size 93.2 x 99.2 mm -> 94.2 x 99.2 mm
- board text added: "ver 0.2"
